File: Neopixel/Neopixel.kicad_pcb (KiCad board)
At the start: 2 copper layers, 22 parts

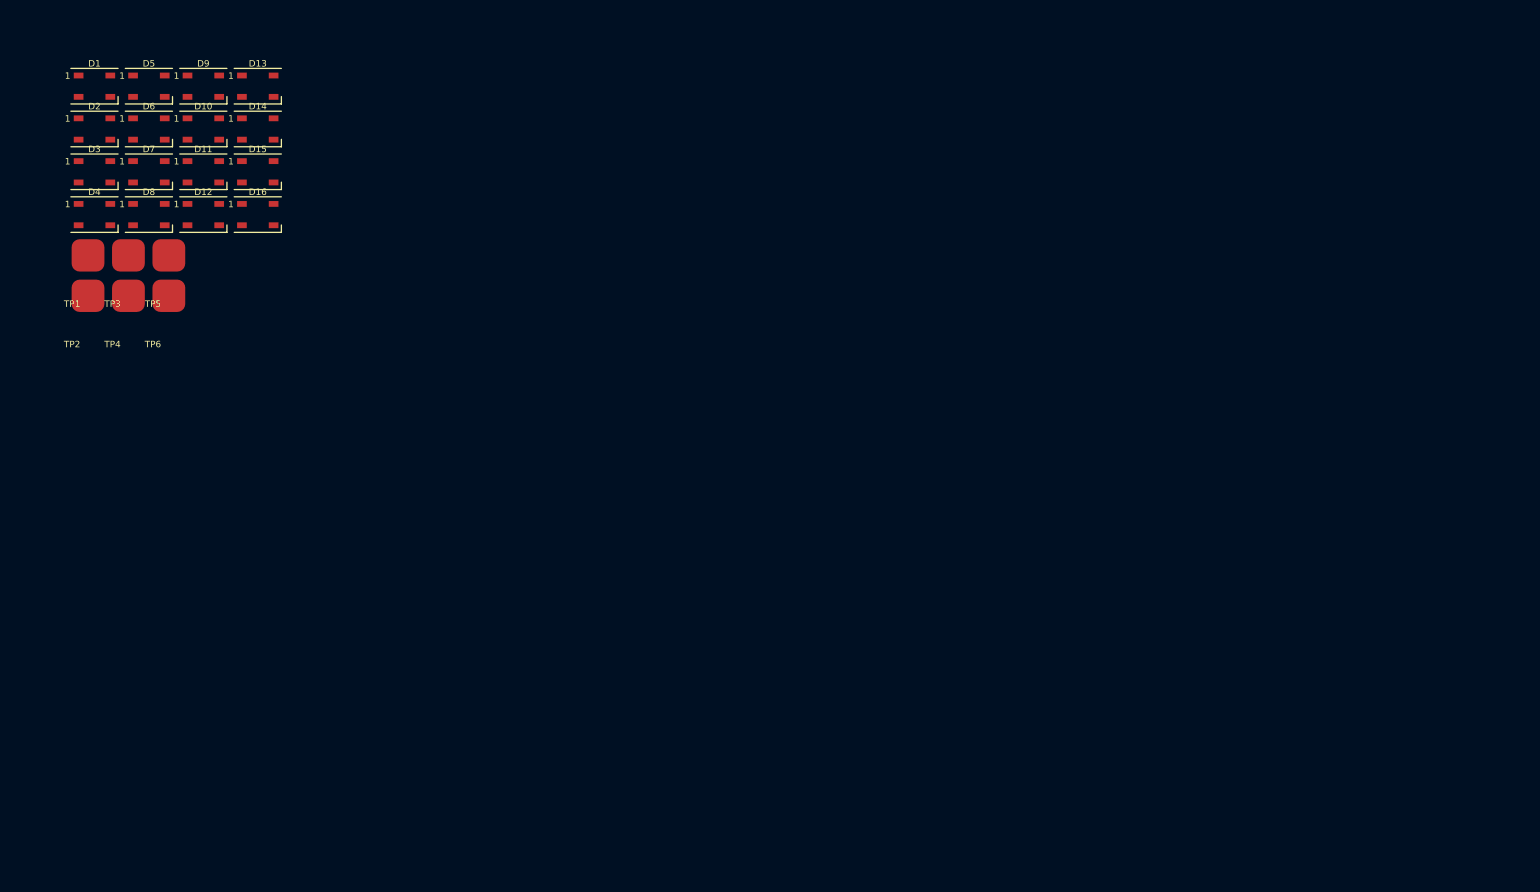
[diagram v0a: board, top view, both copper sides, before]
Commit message: designing
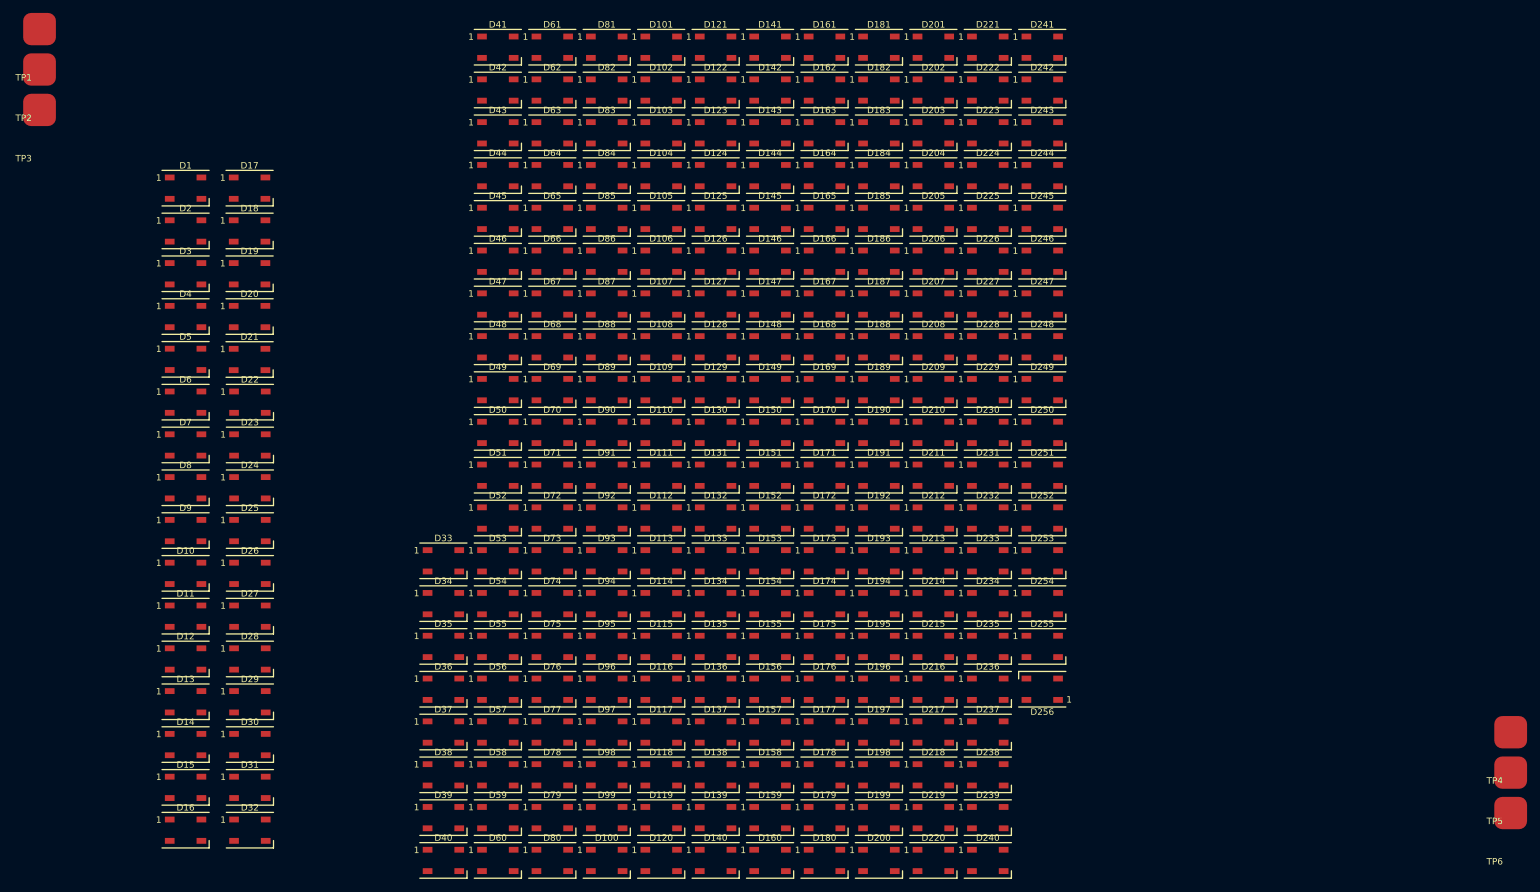
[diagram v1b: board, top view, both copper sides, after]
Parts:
- added D100: WS2812B, LED_SMD:LED_WS2812B_PLCC4_5.0x5.0mm_P3.2mm, F.Cu at (105.2, 147.3)
- added D101: WS2812B, LED_SMD:LED_WS2812B_PLCC4_5.0x5.0mm_P3.2mm, F.Cu at (113.6, 21.6)
- added D102: WS2812B, LED_SMD:LED_WS2812B_PLCC4_5.0x5.0mm_P3.2mm, F.Cu at (113.6, 28.2)
- added D103: WS2812B, LED_SMD:LED_WS2812B_PLCC4_5.0x5.0mm_P3.2mm, F.Cu at (113.6, 34.8)
- added D104: WS2812B, LED_SMD:LED_WS2812B_PLCC4_5.0x5.0mm_P3.2mm, F.Cu at (113.6, 41.4)
- added D105: WS2812B, LED_SMD:LED_WS2812B_PLCC4_5.0x5.0mm_P3.2mm, F.Cu at (113.6, 48.0)
- added D106: WS2812B, LED_SMD:LED_WS2812B_PLCC4_5.0x5.0mm_P3.2mm, F.Cu at (113.6, 54.6)
- added D107: WS2812B, LED_SMD:LED_WS2812B_PLCC4_5.0x5.0mm_P3.2mm, F.Cu at (113.6, 61.3)
- added D108: WS2812B, LED_SMD:LED_WS2812B_PLCC4_5.0x5.0mm_P3.2mm, F.Cu at (113.6, 67.9)
- added D109: WS2812B, LED_SMD:LED_WS2812B_PLCC4_5.0x5.0mm_P3.2mm, F.Cu at (113.6, 74.5)
- added D110: WS2812B, LED_SMD:LED_WS2812B_PLCC4_5.0x5.0mm_P3.2mm, F.Cu at (113.6, 81.1)
- added D111: WS2812B, LED_SMD:LED_WS2812B_PLCC4_5.0x5.0mm_P3.2mm, F.Cu at (113.6, 87.8)
- added D112: WS2812B, LED_SMD:LED_WS2812B_PLCC4_5.0x5.0mm_P3.2mm, F.Cu at (113.6, 94.4)
- added D113: WS2812B, LED_SMD:LED_WS2812B_PLCC4_5.0x5.0mm_P3.2mm, F.Cu at (113.6, 101.0)
- added D114: WS2812B, LED_SMD:LED_WS2812B_PLCC4_5.0x5.0mm_P3.2mm, F.Cu at (113.6, 107.6)
- added D115: WS2812B, LED_SMD:LED_WS2812B_PLCC4_5.0x5.0mm_P3.2mm, F.Cu at (113.6, 114.2)
- added D116: WS2812B, LED_SMD:LED_WS2812B_PLCC4_5.0x5.0mm_P3.2mm, F.Cu at (113.6, 120.8)
- added D117: WS2812B, LED_SMD:LED_WS2812B_PLCC4_5.0x5.0mm_P3.2mm, F.Cu at (113.6, 127.5)
- added D118: WS2812B, LED_SMD:LED_WS2812B_PLCC4_5.0x5.0mm_P3.2mm, F.Cu at (113.6, 134.1)
- added D119: WS2812B, LED_SMD:LED_WS2812B_PLCC4_5.0x5.0mm_P3.2mm, F.Cu at (113.6, 140.7)
- added D120: WS2812B, LED_SMD:LED_WS2812B_PLCC4_5.0x5.0mm_P3.2mm, F.Cu at (113.6, 147.3)
- added D121: WS2812B, LED_SMD:LED_WS2812B_PLCC4_5.0x5.0mm_P3.2mm, F.Cu at (122.0, 21.6)
- added D122: WS2812B, LED_SMD:LED_WS2812B_PLCC4_5.0x5.0mm_P3.2mm, F.Cu at (122.0, 28.2)
- added D123: WS2812B, LED_SMD:LED_WS2812B_PLCC4_5.0x5.0mm_P3.2mm, F.Cu at (122.0, 34.8)
- added D124: WS2812B, LED_SMD:LED_WS2812B_PLCC4_5.0x5.0mm_P3.2mm, F.Cu at (122.0, 41.4)
- added D125: WS2812B, LED_SMD:LED_WS2812B_PLCC4_5.0x5.0mm_P3.2mm, F.Cu at (122.0, 48.0)
- added D126: WS2812B, LED_SMD:LED_WS2812B_PLCC4_5.0x5.0mm_P3.2mm, F.Cu at (122.0, 54.6)
- added D127: WS2812B, LED_SMD:LED_WS2812B_PLCC4_5.0x5.0mm_P3.2mm, F.Cu at (122.0, 61.3)
- added D128: WS2812B, LED_SMD:LED_WS2812B_PLCC4_5.0x5.0mm_P3.2mm, F.Cu at (122.0, 67.9)
- added D129: WS2812B, LED_SMD:LED_WS2812B_PLCC4_5.0x5.0mm_P3.2mm, F.Cu at (122.0, 74.5)
- added D130: WS2812B, LED_SMD:LED_WS2812B_PLCC4_5.0x5.0mm_P3.2mm, F.Cu at (122.0, 81.1)
- added D131: WS2812B, LED_SMD:LED_WS2812B_PLCC4_5.0x5.0mm_P3.2mm, F.Cu at (122.0, 87.8)
- added D132: WS2812B, LED_SMD:LED_WS2812B_PLCC4_5.0x5.0mm_P3.2mm, F.Cu at (122.0, 94.4)
- added D133: WS2812B, LED_SMD:LED_WS2812B_PLCC4_5.0x5.0mm_P3.2mm, F.Cu at (122.0, 101.0)
- added D134: WS2812B, LED_SMD:LED_WS2812B_PLCC4_5.0x5.0mm_P3.2mm, F.Cu at (122.0, 107.6)
- added D135: WS2812B, LED_SMD:LED_WS2812B_PLCC4_5.0x5.0mm_P3.2mm, F.Cu at (122.0, 114.2)
- added D136: WS2812B, LED_SMD:LED_WS2812B_PLCC4_5.0x5.0mm_P3.2mm, F.Cu at (122.0, 120.8)
- added D137: WS2812B, LED_SMD:LED_WS2812B_PLCC4_5.0x5.0mm_P3.2mm, F.Cu at (122.0, 127.5)
- added D138: WS2812B, LED_SMD:LED_WS2812B_PLCC4_5.0x5.0mm_P3.2mm, F.Cu at (122.0, 134.1)
- added D139: WS2812B, LED_SMD:LED_WS2812B_PLCC4_5.0x5.0mm_P3.2mm, F.Cu at (122.0, 140.7)
- added D140: WS2812B, LED_SMD:LED_WS2812B_PLCC4_5.0x5.0mm_P3.2mm, F.Cu at (122.0, 147.3)
- added D141: WS2812B, LED_SMD:LED_WS2812B_PLCC4_5.0x5.0mm_P3.2mm, F.Cu at (130.4, 21.6)
- added D142: WS2812B, LED_SMD:LED_WS2812B_PLCC4_5.0x5.0mm_P3.2mm, F.Cu at (130.4, 28.2)
- added D143: WS2812B, LED_SMD:LED_WS2812B_PLCC4_5.0x5.0mm_P3.2mm, F.Cu at (130.4, 34.8)
- added D144: WS2812B, LED_SMD:LED_WS2812B_PLCC4_5.0x5.0mm_P3.2mm, F.Cu at (130.4, 41.4)
- added D145: WS2812B, LED_SMD:LED_WS2812B_PLCC4_5.0x5.0mm_P3.2mm, F.Cu at (130.4, 48.0)
- added D146: WS2812B, LED_SMD:LED_WS2812B_PLCC4_5.0x5.0mm_P3.2mm, F.Cu at (130.4, 54.6)
- added D147: WS2812B, LED_SMD:LED_WS2812B_PLCC4_5.0x5.0mm_P3.2mm, F.Cu at (130.4, 61.3)
- added D148: WS2812B, LED_SMD:LED_WS2812B_PLCC4_5.0x5.0mm_P3.2mm, F.Cu at (130.4, 67.9)
- added D149: WS2812B, LED_SMD:LED_WS2812B_PLCC4_5.0x5.0mm_P3.2mm, F.Cu at (130.4, 74.5)
- added D150: WS2812B, LED_SMD:LED_WS2812B_PLCC4_5.0x5.0mm_P3.2mm, F.Cu at (130.4, 81.1)
- added D151: WS2812B, LED_SMD:LED_WS2812B_PLCC4_5.0x5.0mm_P3.2mm, F.Cu at (130.4, 87.8)
- added D152: WS2812B, LED_SMD:LED_WS2812B_PLCC4_5.0x5.0mm_P3.2mm, F.Cu at (130.4, 94.4)
- added D153: WS2812B, LED_SMD:LED_WS2812B_PLCC4_5.0x5.0mm_P3.2mm, F.Cu at (130.4, 101.0)
- added D154: WS2812B, LED_SMD:LED_WS2812B_PLCC4_5.0x5.0mm_P3.2mm, F.Cu at (130.4, 107.6)
- added D155: WS2812B, LED_SMD:LED_WS2812B_PLCC4_5.0x5.0mm_P3.2mm, F.Cu at (130.4, 114.2)
- added D156: WS2812B, LED_SMD:LED_WS2812B_PLCC4_5.0x5.0mm_P3.2mm, F.Cu at (130.4, 120.8)
- added D157: WS2812B, LED_SMD:LED_WS2812B_PLCC4_5.0x5.0mm_P3.2mm, F.Cu at (130.4, 127.5)
- added D158: WS2812B, LED_SMD:LED_WS2812B_PLCC4_5.0x5.0mm_P3.2mm, F.Cu at (130.4, 134.1)
- added D159: WS2812B, LED_SMD:LED_WS2812B_PLCC4_5.0x5.0mm_P3.2mm, F.Cu at (130.4, 140.7)
- added D160: WS2812B, LED_SMD:LED_WS2812B_PLCC4_5.0x5.0mm_P3.2mm, F.Cu at (130.4, 147.3)
- added D161: WS2812B, LED_SMD:LED_WS2812B_PLCC4_5.0x5.0mm_P3.2mm, F.Cu at (138.9, 21.6)
- added D162: WS2812B, LED_SMD:LED_WS2812B_PLCC4_5.0x5.0mm_P3.2mm, F.Cu at (138.9, 28.2)
- added D163: WS2812B, LED_SMD:LED_WS2812B_PLCC4_5.0x5.0mm_P3.2mm, F.Cu at (138.9, 34.8)
- added D164: WS2812B, LED_SMD:LED_WS2812B_PLCC4_5.0x5.0mm_P3.2mm, F.Cu at (138.9, 41.4)
- added D165: WS2812B, LED_SMD:LED_WS2812B_PLCC4_5.0x5.0mm_P3.2mm, F.Cu at (138.9, 48.0)
- added D166: WS2812B, LED_SMD:LED_WS2812B_PLCC4_5.0x5.0mm_P3.2mm, F.Cu at (138.9, 54.6)
- added D167: WS2812B, LED_SMD:LED_WS2812B_PLCC4_5.0x5.0mm_P3.2mm, F.Cu at (138.9, 61.3)
- added D168: WS2812B, LED_SMD:LED_WS2812B_PLCC4_5.0x5.0mm_P3.2mm, F.Cu at (138.9, 67.9)
- added D169: WS2812B, LED_SMD:LED_WS2812B_PLCC4_5.0x5.0mm_P3.2mm, F.Cu at (138.9, 74.5)
- added D17: WS2812B, LED_SMD:LED_WS2812B_PLCC4_5.0x5.0mm_P3.2mm, F.Cu at (50.0, 43.4)
- added D170: WS2812B, LED_SMD:LED_WS2812B_PLCC4_5.0x5.0mm_P3.2mm, F.Cu at (138.9, 81.1)
- added D171: WS2812B, LED_SMD:LED_WS2812B_PLCC4_5.0x5.0mm_P3.2mm, F.Cu at (138.9, 87.8)
- added D172: WS2812B, LED_SMD:LED_WS2812B_PLCC4_5.0x5.0mm_P3.2mm, F.Cu at (138.9, 94.4)
- added D173: WS2812B, LED_SMD:LED_WS2812B_PLCC4_5.0x5.0mm_P3.2mm, F.Cu at (138.9, 101.0)
- added D174: WS2812B, LED_SMD:LED_WS2812B_PLCC4_5.0x5.0mm_P3.2mm, F.Cu at (138.9, 107.6)
- added D175: WS2812B, LED_SMD:LED_WS2812B_PLCC4_5.0x5.0mm_P3.2mm, F.Cu at (138.9, 114.2)
- added D176: WS2812B, LED_SMD:LED_WS2812B_PLCC4_5.0x5.0mm_P3.2mm, F.Cu at (138.9, 120.8)
- added D177: WS2812B, LED_SMD:LED_WS2812B_PLCC4_5.0x5.0mm_P3.2mm, F.Cu at (138.9, 127.5)
- added D178: WS2812B, LED_SMD:LED_WS2812B_PLCC4_5.0x5.0mm_P3.2mm, F.Cu at (138.9, 134.1)
- added D179: WS2812B, LED_SMD:LED_WS2812B_PLCC4_5.0x5.0mm_P3.2mm, F.Cu at (138.9, 140.7)
- added D18: WS2812B, LED_SMD:LED_WS2812B_PLCC4_5.0x5.0mm_P3.2mm, F.Cu at (50.0, 50.0)
- added D180: WS2812B, LED_SMD:LED_WS2812B_PLCC4_5.0x5.0mm_P3.2mm, F.Cu at (138.9, 147.3)
- added D181: WS2812B, LED_SMD:LED_WS2812B_PLCC4_5.0x5.0mm_P3.2mm, F.Cu at (147.3, 21.6)
- added D182: WS2812B, LED_SMD:LED_WS2812B_PLCC4_5.0x5.0mm_P3.2mm, F.Cu at (147.3, 28.2)
- added D183: WS2812B, LED_SMD:LED_WS2812B_PLCC4_5.0x5.0mm_P3.2mm, F.Cu at (147.3, 34.8)
- added D184: WS2812B, LED_SMD:LED_WS2812B_PLCC4_5.0x5.0mm_P3.2mm, F.Cu at (147.3, 41.4)
- added D185: WS2812B, LED_SMD:LED_WS2812B_PLCC4_5.0x5.0mm_P3.2mm, F.Cu at (147.3, 48.0)
- added D186: WS2812B, LED_SMD:LED_WS2812B_PLCC4_5.0x5.0mm_P3.2mm, F.Cu at (147.3, 54.6)
- added D187: WS2812B, LED_SMD:LED_WS2812B_PLCC4_5.0x5.0mm_P3.2mm, F.Cu at (147.3, 61.3)
- added D188: WS2812B, LED_SMD:LED_WS2812B_PLCC4_5.0x5.0mm_P3.2mm, F.Cu at (147.3, 67.9)
- added D189: WS2812B, LED_SMD:LED_WS2812B_PLCC4_5.0x5.0mm_P3.2mm, F.Cu at (147.3, 74.5)
- added D19: WS2812B, LED_SMD:LED_WS2812B_PLCC4_5.0x5.0mm_P3.2mm, F.Cu at (50.0, 56.6)
- added D190: WS2812B, LED_SMD:LED_WS2812B_PLCC4_5.0x5.0mm_P3.2mm, F.Cu at (147.3, 81.1)
- added D191: WS2812B, LED_SMD:LED_WS2812B_PLCC4_5.0x5.0mm_P3.2mm, F.Cu at (147.3, 87.8)
- added D192: WS2812B, LED_SMD:LED_WS2812B_PLCC4_5.0x5.0mm_P3.2mm, F.Cu at (147.3, 94.4)
- added D193: WS2812B, LED_SMD:LED_WS2812B_PLCC4_5.0x5.0mm_P3.2mm, F.Cu at (147.3, 101.0)
- added D194: WS2812B, LED_SMD:LED_WS2812B_PLCC4_5.0x5.0mm_P3.2mm, F.Cu at (147.3, 107.6)
- added D195: WS2812B, LED_SMD:LED_WS2812B_PLCC4_5.0x5.0mm_P3.2mm, F.Cu at (147.3, 114.2)
- added D196: WS2812B, LED_SMD:LED_WS2812B_PLCC4_5.0x5.0mm_P3.2mm, F.Cu at (147.3, 120.8)
- added D197: WS2812B, LED_SMD:LED_WS2812B_PLCC4_5.0x5.0mm_P3.2mm, F.Cu at (147.3, 127.5)
- added D198: WS2812B, LED_SMD:LED_WS2812B_PLCC4_5.0x5.0mm_P3.2mm, F.Cu at (147.3, 134.1)
- added D199: WS2812B, LED_SMD:LED_WS2812B_PLCC4_5.0x5.0mm_P3.2mm, F.Cu at (147.3, 140.7)
- added D20: WS2812B, LED_SMD:LED_WS2812B_PLCC4_5.0x5.0mm_P3.2mm, F.Cu at (50.0, 63.2)
- added D200: WS2812B, LED_SMD:LED_WS2812B_PLCC4_5.0x5.0mm_P3.2mm, F.Cu at (147.3, 147.3)
- added D201: WS2812B, LED_SMD:LED_WS2812B_PLCC4_5.0x5.0mm_P3.2mm, F.Cu at (155.7, 21.6)
- added D202: WS2812B, LED_SMD:LED_WS2812B_PLCC4_5.0x5.0mm_P3.2mm, F.Cu at (155.7, 28.2)
- added D203: WS2812B, LED_SMD:LED_WS2812B_PLCC4_5.0x5.0mm_P3.2mm, F.Cu at (155.7, 34.8)
- added D204: WS2812B, LED_SMD:LED_WS2812B_PLCC4_5.0x5.0mm_P3.2mm, F.Cu at (155.7, 41.4)
- added D205: WS2812B, LED_SMD:LED_WS2812B_PLCC4_5.0x5.0mm_P3.2mm, F.Cu at (155.7, 48.0)
- added D206: WS2812B, LED_SMD:LED_WS2812B_PLCC4_5.0x5.0mm_P3.2mm, F.Cu at (155.7, 54.6)
- added D207: WS2812B, LED_SMD:LED_WS2812B_PLCC4_5.0x5.0mm_P3.2mm, F.Cu at (155.7, 61.3)
- added D208: WS2812B, LED_SMD:LED_WS2812B_PLCC4_5.0x5.0mm_P3.2mm, F.Cu at (155.7, 67.9)
- added D209: WS2812B, LED_SMD:LED_WS2812B_PLCC4_5.0x5.0mm_P3.2mm, F.Cu at (155.7, 74.5)
- added D21: WS2812B, LED_SMD:LED_WS2812B_PLCC4_5.0x5.0mm_P3.2mm, F.Cu at (50.0, 69.8)
- added D210: WS2812B, LED_SMD:LED_WS2812B_PLCC4_5.0x5.0mm_P3.2mm, F.Cu at (155.7, 81.1)
- added D211: WS2812B, LED_SMD:LED_WS2812B_PLCC4_5.0x5.0mm_P3.2mm, F.Cu at (155.7, 87.8)
- added D212: WS2812B, LED_SMD:LED_WS2812B_PLCC4_5.0x5.0mm_P3.2mm, F.Cu at (155.7, 94.4)
- added D213: WS2812B, LED_SMD:LED_WS2812B_PLCC4_5.0x5.0mm_P3.2mm, F.Cu at (155.7, 101.0)
- added D214: WS2812B, LED_SMD:LED_WS2812B_PLCC4_5.0x5.0mm_P3.2mm, F.Cu at (155.7, 107.6)
- added D215: WS2812B, LED_SMD:LED_WS2812B_PLCC4_5.0x5.0mm_P3.2mm, F.Cu at (155.7, 114.2)
- added D216: WS2812B, LED_SMD:LED_WS2812B_PLCC4_5.0x5.0mm_P3.2mm, F.Cu at (155.7, 120.8)
- added D217: WS2812B, LED_SMD:LED_WS2812B_PLCC4_5.0x5.0mm_P3.2mm, F.Cu at (155.7, 127.5)
- added D218: WS2812B, LED_SMD:LED_WS2812B_PLCC4_5.0x5.0mm_P3.2mm, F.Cu at (155.7, 134.1)
- added D219: WS2812B, LED_SMD:LED_WS2812B_PLCC4_5.0x5.0mm_P3.2mm, F.Cu at (155.7, 140.7)
- added D22: WS2812B, LED_SMD:LED_WS2812B_PLCC4_5.0x5.0mm_P3.2mm, F.Cu at (50.0, 76.5)
- added D220: WS2812B, LED_SMD:LED_WS2812B_PLCC4_5.0x5.0mm_P3.2mm, F.Cu at (155.7, 147.3)
- added D221: WS2812B, LED_SMD:LED_WS2812B_PLCC4_5.0x5.0mm_P3.2mm, F.Cu at (164.1, 21.6)
- added D222: WS2812B, LED_SMD:LED_WS2812B_PLCC4_5.0x5.0mm_P3.2mm, F.Cu at (164.1, 28.2)
- added D223: WS2812B, LED_SMD:LED_WS2812B_PLCC4_5.0x5.0mm_P3.2mm, F.Cu at (164.1, 34.8)
- added D224: WS2812B, LED_SMD:LED_WS2812B_PLCC4_5.0x5.0mm_P3.2mm, F.Cu at (164.1, 41.4)
- added D225: WS2812B, LED_SMD:LED_WS2812B_PLCC4_5.0x5.0mm_P3.2mm, F.Cu at (164.1, 48.0)
- added D226: WS2812B, LED_SMD:LED_WS2812B_PLCC4_5.0x5.0mm_P3.2mm, F.Cu at (164.1, 54.6)
- added D227: WS2812B, LED_SMD:LED_WS2812B_PLCC4_5.0x5.0mm_P3.2mm, F.Cu at (164.1, 61.3)
- added D228: WS2812B, LED_SMD:LED_WS2812B_PLCC4_5.0x5.0mm_P3.2mm, F.Cu at (164.1, 67.9)
- added D229: WS2812B, LED_SMD:LED_WS2812B_PLCC4_5.0x5.0mm_P3.2mm, F.Cu at (164.1, 74.5)
- added D23: WS2812B, LED_SMD:LED_WS2812B_PLCC4_5.0x5.0mm_P3.2mm, F.Cu at (50.0, 83.1)
- added D230: WS2812B, LED_SMD:LED_WS2812B_PLCC4_5.0x5.0mm_P3.2mm, F.Cu at (164.1, 81.1)
- added D231: WS2812B, LED_SMD:LED_WS2812B_PLCC4_5.0x5.0mm_P3.2mm, F.Cu at (164.1, 87.8)
- added D232: WS2812B, LED_SMD:LED_WS2812B_PLCC4_5.0x5.0mm_P3.2mm, F.Cu at (164.1, 94.4)
- added D233: WS2812B, LED_SMD:LED_WS2812B_PLCC4_5.0x5.0mm_P3.2mm, F.Cu at (164.1, 101.0)
- added D234: WS2812B, LED_SMD:LED_WS2812B_PLCC4_5.0x5.0mm_P3.2mm, F.Cu at (164.1, 107.6)
- added D235: WS2812B, LED_SMD:LED_WS2812B_PLCC4_5.0x5.0mm_P3.2mm, F.Cu at (164.1, 114.2)
- added D236: WS2812B, LED_SMD:LED_WS2812B_PLCC4_5.0x5.0mm_P3.2mm, F.Cu at (164.1, 120.8)
- added D237: WS2812B, LED_SMD:LED_WS2812B_PLCC4_5.0x5.0mm_P3.2mm, F.Cu at (164.1, 127.5)
- added D238: WS2812B, LED_SMD:LED_WS2812B_PLCC4_5.0x5.0mm_P3.2mm, F.Cu at (164.1, 134.1)
- added D239: WS2812B, LED_SMD:LED_WS2812B_PLCC4_5.0x5.0mm_P3.2mm, F.Cu at (164.1, 140.7)
- added D24: WS2812B, LED_SMD:LED_WS2812B_PLCC4_5.0x5.0mm_P3.2mm, F.Cu at (50.0, 89.7)
- added D240: WS2812B, LED_SMD:LED_WS2812B_PLCC4_5.0x5.0mm_P3.2mm, F.Cu at (164.1, 147.3)
- added D241: WS2812B, LED_SMD:LED_WS2812B_PLCC4_5.0x5.0mm_P3.2mm, F.Cu at (172.6, 21.6)
- added D242: WS2812B, LED_SMD:LED_WS2812B_PLCC4_5.0x5.0mm_P3.2mm, F.Cu at (172.6, 28.2)
- added D243: WS2812B, LED_SMD:LED_WS2812B_PLCC4_5.0x5.0mm_P3.2mm, F.Cu at (172.6, 34.8)
- added D244: WS2812B, LED_SMD:LED_WS2812B_PLCC4_5.0x5.0mm_P3.2mm, F.Cu at (172.6, 41.4)
- added D245: WS2812B, LED_SMD:LED_WS2812B_PLCC4_5.0x5.0mm_P3.2mm, F.Cu at (172.6, 48.0)
- added D246: WS2812B, LED_SMD:LED_WS2812B_PLCC4_5.0x5.0mm_P3.2mm, F.Cu at (172.6, 54.6)
- added D247: WS2812B, LED_SMD:LED_WS2812B_PLCC4_5.0x5.0mm_P3.2mm, F.Cu at (172.6, 61.3)
- added D248: WS2812B, LED_SMD:LED_WS2812B_PLCC4_5.0x5.0mm_P3.2mm, F.Cu at (172.6, 67.9)
- added D249: WS2812B, LED_SMD:LED_WS2812B_PLCC4_5.0x5.0mm_P3.2mm, F.Cu at (172.6, 74.5)
- added D25: WS2812B, LED_SMD:LED_WS2812B_PLCC4_5.0x5.0mm_P3.2mm, F.Cu at (50.0, 96.3)
- added D250: WS2812B, LED_SMD:LED_WS2812B_PLCC4_5.0x5.0mm_P3.2mm, F.Cu at (172.6, 81.1)
- added D251: WS2812B, LED_SMD:LED_WS2812B_PLCC4_5.0x5.0mm_P3.2mm, F.Cu at (172.6, 87.8)
- added D252: WS2812B, LED_SMD:LED_WS2812B_PLCC4_5.0x5.0mm_P3.2mm, F.Cu at (172.6, 94.4)
- added D253: WS2812B, LED_SMD:LED_WS2812B_PLCC4_5.0x5.0mm_P3.2mm, F.Cu at (172.6, 101.0)
- added D254: WS2812B, LED_SMD:LED_WS2812B_PLCC4_5.0x5.0mm_P3.2mm, F.Cu at (172.6, 107.6)
- added D255: WS2812B, LED_SMD:LED_WS2812B_PLCC4_5.0x5.0mm_P3.2mm, F.Cu at (172.6, 114.2)
- added D256: WS2812B, LED_SMD:LED_WS2812B_PLCC4_5.0x5.0mm_P3.2mm, F.Cu at (172.6, 120.8)
- added D26: WS2812B, LED_SMD:LED_WS2812B_PLCC4_5.0x5.0mm_P3.2mm, F.Cu at (50.0, 102.9)
- added D27: WS2812B, LED_SMD:LED_WS2812B_PLCC4_5.0x5.0mm_P3.2mm, F.Cu at (50.0, 109.5)
- added D28: WS2812B, LED_SMD:LED_WS2812B_PLCC4_5.0x5.0mm_P3.2mm, F.Cu at (50.0, 116.2)
- added D29: WS2812B, LED_SMD:LED_WS2812B_PLCC4_5.0x5.0mm_P3.2mm, F.Cu at (50.0, 122.8)
- added D30: WS2812B, LED_SMD:LED_WS2812B_PLCC4_5.0x5.0mm_P3.2mm, F.Cu at (50.0, 129.4)
- added D31: WS2812B, LED_SMD:LED_WS2812B_PLCC4_5.0x5.0mm_P3.2mm, F.Cu at (50.0, 136.0)
- added D32: WS2812B, LED_SMD:LED_WS2812B_PLCC4_5.0x5.0mm_P3.2mm, F.Cu at (50.0, 142.7)
- added D33: WS2812B, LED_SMD:LED_WS2812B_PLCC4_5.0x5.0mm_P3.2mm, F.Cu at (79.9, 101.0)
- added D34: WS2812B, LED_SMD:LED_WS2812B_PLCC4_5.0x5.0mm_P3.2mm, F.Cu at (79.9, 107.6)
- added D35: WS2812B, LED_SMD:LED_WS2812B_PLCC4_5.0x5.0mm_P3.2mm, F.Cu at (79.9, 114.2)
- added D36: WS2812B, LED_SMD:LED_WS2812B_PLCC4_5.0x5.0mm_P3.2mm, F.Cu at (79.9, 120.8)
- added D37: WS2812B, LED_SMD:LED_WS2812B_PLCC4_5.0x5.0mm_P3.2mm, F.Cu at (79.9, 127.5)
- added D38: WS2812B, LED_SMD:LED_WS2812B_PLCC4_5.0x5.0mm_P3.2mm, F.Cu at (79.9, 134.1)
- added D39: WS2812B, LED_SMD:LED_WS2812B_PLCC4_5.0x5.0mm_P3.2mm, F.Cu at (79.9, 140.7)
- added D40: WS2812B, LED_SMD:LED_WS2812B_PLCC4_5.0x5.0mm_P3.2mm, F.Cu at (79.9, 147.3)
- added D41: WS2812B, LED_SMD:LED_WS2812B_PLCC4_5.0x5.0mm_P3.2mm, F.Cu at (88.3, 21.6)
- added D42: WS2812B, LED_SMD:LED_WS2812B_PLCC4_5.0x5.0mm_P3.2mm, F.Cu at (88.3, 28.2)
- added D43: WS2812B, LED_SMD:LED_WS2812B_PLCC4_5.0x5.0mm_P3.2mm, F.Cu at (88.3, 34.8)
- added D44: WS2812B, LED_SMD:LED_WS2812B_PLCC4_5.0x5.0mm_P3.2mm, F.Cu at (88.3, 41.4)
- added D45: WS2812B, LED_SMD:LED_WS2812B_PLCC4_5.0x5.0mm_P3.2mm, F.Cu at (88.3, 48.0)
- added D46: WS2812B, LED_SMD:LED_WS2812B_PLCC4_5.0x5.0mm_P3.2mm, F.Cu at (88.3, 54.6)
- added D47: WS2812B, LED_SMD:LED_WS2812B_PLCC4_5.0x5.0mm_P3.2mm, F.Cu at (88.3, 61.3)
- added D48: WS2812B, LED_SMD:LED_WS2812B_PLCC4_5.0x5.0mm_P3.2mm, F.Cu at (88.3, 67.9)
- added D49: WS2812B, LED_SMD:LED_WS2812B_PLCC4_5.0x5.0mm_P3.2mm, F.Cu at (88.3, 74.5)
- added D50: WS2812B, LED_SMD:LED_WS2812B_PLCC4_5.0x5.0mm_P3.2mm, F.Cu at (88.3, 81.1)
- added D51: WS2812B, LED_SMD:LED_WS2812B_PLCC4_5.0x5.0mm_P3.2mm, F.Cu at (88.3, 87.8)
- added D52: WS2812B, LED_SMD:LED_WS2812B_PLCC4_5.0x5.0mm_P3.2mm, F.Cu at (88.3, 94.4)
- added D53: WS2812B, LED_SMD:LED_WS2812B_PLCC4_5.0x5.0mm_P3.2mm, F.Cu at (88.3, 101.0)
- added D54: WS2812B, LED_SMD:LED_WS2812B_PLCC4_5.0x5.0mm_P3.2mm, F.Cu at (88.3, 107.6)
- added D55: WS2812B, LED_SMD:LED_WS2812B_PLCC4_5.0x5.0mm_P3.2mm, F.Cu at (88.3, 114.2)
- added D56: WS2812B, LED_SMD:LED_WS2812B_PLCC4_5.0x5.0mm_P3.2mm, F.Cu at (88.3, 120.8)
- added D57: WS2812B, LED_SMD:LED_WS2812B_PLCC4_5.0x5.0mm_P3.2mm, F.Cu at (88.3, 127.5)
- added D58: WS2812B, LED_SMD:LED_WS2812B_PLCC4_5.0x5.0mm_P3.2mm, F.Cu at (88.3, 134.1)
- added D59: WS2812B, LED_SMD:LED_WS2812B_PLCC4_5.0x5.0mm_P3.2mm, F.Cu at (88.3, 140.7)
- added D60: WS2812B, LED_SMD:LED_WS2812B_PLCC4_5.0x5.0mm_P3.2mm, F.Cu at (88.3, 147.3)
- added D61: WS2812B, LED_SMD:LED_WS2812B_PLCC4_5.0x5.0mm_P3.2mm, F.Cu at (96.8, 21.6)
- added D62: WS2812B, LED_SMD:LED_WS2812B_PLCC4_5.0x5.0mm_P3.2mm, F.Cu at (96.8, 28.2)
- added D63: WS2812B, LED_SMD:LED_WS2812B_PLCC4_5.0x5.0mm_P3.2mm, F.Cu at (96.8, 34.8)
- added D64: WS2812B, LED_SMD:LED_WS2812B_PLCC4_5.0x5.0mm_P3.2mm, F.Cu at (96.8, 41.4)
- added D65: WS2812B, LED_SMD:LED_WS2812B_PLCC4_5.0x5.0mm_P3.2mm, F.Cu at (96.8, 48.0)
- added D66: WS2812B, LED_SMD:LED_WS2812B_PLCC4_5.0x5.0mm_P3.2mm, F.Cu at (96.8, 54.6)
- added D67: WS2812B, LED_SMD:LED_WS2812B_PLCC4_5.0x5.0mm_P3.2mm, F.Cu at (96.8, 61.3)
- added D68: WS2812B, LED_SMD:LED_WS2812B_PLCC4_5.0x5.0mm_P3.2mm, F.Cu at (96.8, 67.9)
- added D69: WS2812B, LED_SMD:LED_WS2812B_PLCC4_5.0x5.0mm_P3.2mm, F.Cu at (96.8, 74.5)
- added D70: WS2812B, LED_SMD:LED_WS2812B_PLCC4_5.0x5.0mm_P3.2mm, F.Cu at (96.8, 81.1)
- added D71: WS2812B, LED_SMD:LED_WS2812B_PLCC4_5.0x5.0mm_P3.2mm, F.Cu at (96.8, 87.8)
- added D72: WS2812B, LED_SMD:LED_WS2812B_PLCC4_5.0x5.0mm_P3.2mm, F.Cu at (96.8, 94.4)
- added D73: WS2812B, LED_SMD:LED_WS2812B_PLCC4_5.0x5.0mm_P3.2mm, F.Cu at (96.8, 101.0)
- added D74: WS2812B, LED_SMD:LED_WS2812B_PLCC4_5.0x5.0mm_P3.2mm, F.Cu at (96.8, 107.6)
- added D75: WS2812B, LED_SMD:LED_WS2812B_PLCC4_5.0x5.0mm_P3.2mm, F.Cu at (96.8, 114.2)
- added D76: WS2812B, LED_SMD:LED_WS2812B_PLCC4_5.0x5.0mm_P3.2mm, F.Cu at (96.8, 120.8)
- added D77: WS2812B, LED_SMD:LED_WS2812B_PLCC4_5.0x5.0mm_P3.2mm, F.Cu at (96.8, 127.5)
- added D78: WS2812B, LED_SMD:LED_WS2812B_PLCC4_5.0x5.0mm_P3.2mm, F.Cu at (96.8, 134.1)
- added D79: WS2812B, LED_SMD:LED_WS2812B_PLCC4_5.0x5.0mm_P3.2mm, F.Cu at (96.8, 140.7)
- added D80: WS2812B, LED_SMD:LED_WS2812B_PLCC4_5.0x5.0mm_P3.2mm, F.Cu at (96.8, 147.3)
- added D81: WS2812B, LED_SMD:LED_WS2812B_PLCC4_5.0x5.0mm_P3.2mm, F.Cu at (105.2, 21.6)
- added D82: WS2812B, LED_SMD:LED_WS2812B_PLCC4_5.0x5.0mm_P3.2mm, F.Cu at (105.2, 28.2)
- added D83: WS2812B, LED_SMD:LED_WS2812B_PLCC4_5.0x5.0mm_P3.2mm, F.Cu at (105.2, 34.8)
- added D84: WS2812B, LED_SMD:LED_WS2812B_PLCC4_5.0x5.0mm_P3.2mm, F.Cu at (105.2, 41.4)
- added D85: WS2812B, LED_SMD:LED_WS2812B_PLCC4_5.0x5.0mm_P3.2mm, F.Cu at (105.2, 48.0)
- added D86: WS2812B, LED_SMD:LED_WS2812B_PLCC4_5.0x5.0mm_P3.2mm, F.Cu at (105.2, 54.6)
- added D87: WS2812B, LED_SMD:LED_WS2812B_PLCC4_5.0x5.0mm_P3.2mm, F.Cu at (105.2, 61.3)
- added D88: WS2812B, LED_SMD:LED_WS2812B_PLCC4_5.0x5.0mm_P3.2mm, F.Cu at (105.2, 67.9)
- added D89: WS2812B, LED_SMD:LED_WS2812B_PLCC4_5.0x5.0mm_P3.2mm, F.Cu at (105.2, 74.5)
- added D90: WS2812B, LED_SMD:LED_WS2812B_PLCC4_5.0x5.0mm_P3.2mm, F.Cu at (105.2, 81.1)
- added D91: WS2812B, LED_SMD:LED_WS2812B_PLCC4_5.0x5.0mm_P3.2mm, F.Cu at (105.2, 87.8)
- added D92: WS2812B, LED_SMD:LED_WS2812B_PLCC4_5.0x5.0mm_P3.2mm, F.Cu at (105.2, 94.4)
- added D93: WS2812B, LED_SMD:LED_WS2812B_PLCC4_5.0x5.0mm_P3.2mm, F.Cu at (105.2, 101.0)
- added D94: WS2812B, LED_SMD:LED_WS2812B_PLCC4_5.0x5.0mm_P3.2mm, F.Cu at (105.2, 107.6)
- added D95: WS2812B, LED_SMD:LED_WS2812B_PLCC4_5.0x5.0mm_P3.2mm, F.Cu at (105.2, 114.2)
- added D96: WS2812B, LED_SMD:LED_WS2812B_PLCC4_5.0x5.0mm_P3.2mm, F.Cu at (105.2, 120.8)
- added D97: WS2812B, LED_SMD:LED_WS2812B_PLCC4_5.0x5.0mm_P3.2mm, F.Cu at (105.2, 127.5)
- added D98: WS2812B, LED_SMD:LED_WS2812B_PLCC4_5.0x5.0mm_P3.2mm, F.Cu at (105.2, 134.1)
- added D99: WS2812B, LED_SMD:LED_WS2812B_PLCC4_5.0x5.0mm_P3.2mm, F.Cu at (105.2, 140.7)
- moved TP4 224.2 mm to (242.5, 130.0)
- moved TP5 222.4 mm to (242.5, 136.2)
- moved TP6 222.4 mm to (242.5, 142.5)
- moved D13 95.9 mm to (40.0, 122.8)
- moved D15 95.9 mm to (40.0, 136.0)
- moved D16 95.9 mm to (40.0, 142.7)
- moved D14 95.9 mm to (40.0, 129.4)
- moved D10 68.8 mm to (40.0, 102.9)
- moved D12 68.8 mm to (40.0, 116.2)
- moved D9 68.8 mm to (40.0, 96.3)
- moved D11 68.8 mm to (40.0, 109.5)
- moved D5 42.6 mm to (40.0, 69.8)
- moved D6 42.6 mm to (40.0, 76.5)
- moved D8 42.6 mm to (40.0, 89.7)
- moved D7 42.6 mm to (40.0, 83.1)
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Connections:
- TP4 pad 1: GND -> +5V
- TP5 pad 1: +5V -> GND
- TP6 pad 1: Net-(D16-DOUT) -> unconnected-(TP6-Pad1)

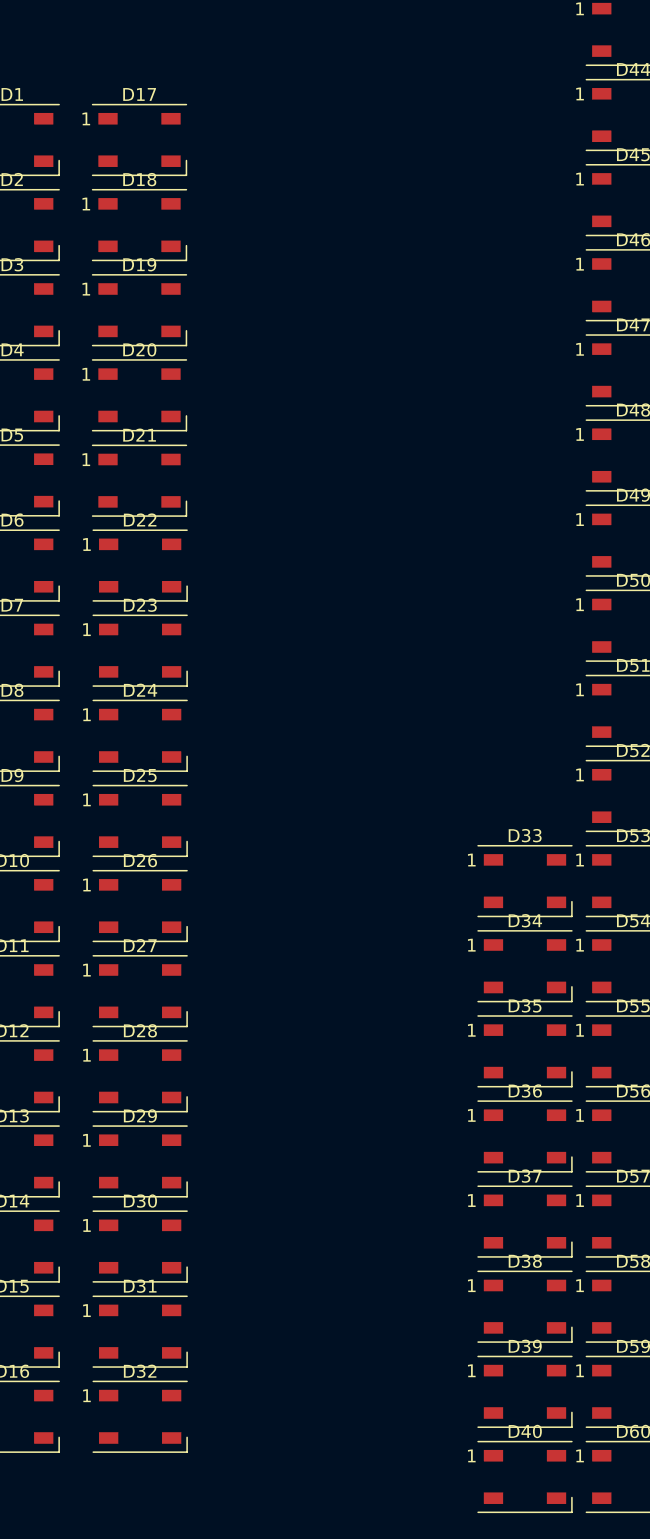
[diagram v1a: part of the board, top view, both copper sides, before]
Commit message: designing
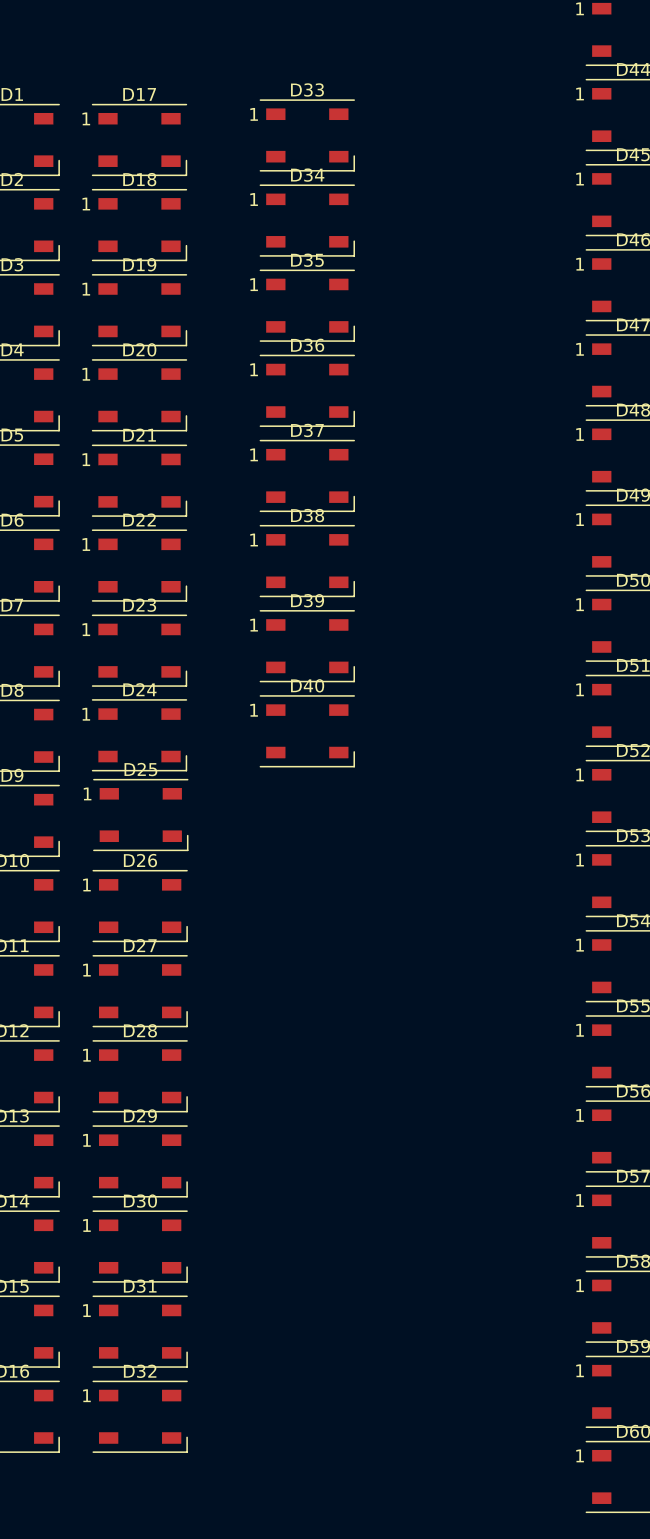
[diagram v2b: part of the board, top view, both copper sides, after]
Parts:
- moved D38 60.4 mm to (63.0, 76.1)
- moved D39 60.4 mm to (63.0, 82.7)
- moved D40 60.4 mm to (63.0, 89.3)
- moved D34 60.4 mm to (63.0, 49.6)
- moved D35 60.4 mm to (63.0, 56.2)
- moved D33 60.4 mm to (63.0, 43.0)
- moved D36 60.4 mm to (63.0, 62.9)
- moved D37 60.4 mm to (63.0, 69.5)
- moved D25 0.46 mm to (50.0, 95.8)
- moved D24 0.06 mm to (50.0, 89.7)
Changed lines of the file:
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@@
 	(footprint "LED_SMD:LED_WS2812B_PLCC4_5.0x5.0mm_P3.2mm"
 		(layer "F.Cu")
-		(at 79.93 120.85)
+		(at 63 62.86)
 		(descr "5.0mm x 5.0mm Addressable RGB LED NeoPixel, https://cdn-shop.adafruit.com/datasheets/WS2812B.pdf")
 		(tags "LED RGB NeoPixel PLCC-4 5050")
@@
 	(footprint "LED_SMD:LED_WS2812B_PLCC4_5.0x5.0mm_P3.2mm"
 		(layer "F.Cu")
-		(at 79.93 114.23)
+		(at 63 56.24)
 		(descr "5.0mm x 5.0mm Addressable RGB LED NeoPixel, https://cdn-shop.adafruit.com/datasheets/WS2812B.pdf")
 		(tags "LED RGB NeoPixel PLCC-4 5050")
@@
 	(footprint "LED_SMD:LED_WS2812B_PLCC4_5.0x5.0mm_P3.2mm"
 		(layer "F.Cu")
-		(at 50 83.07)
+		(at 49.95 83.07)
 		(descr "5.0mm x 5.0mm Addressable RGB LED NeoPixel, https://cdn-shop.adafruit.com/datasheets/WS2812B.pdf")
 		(tags "LED RGB NeoPixel PLCC-4 5050")
@@
 	(footprint "LED_SMD:LED_WS2812B_PLCC4_5.0x5.0mm_P3.2mm"
 		(layer "F.Cu")
-		(at 79.93 140.71)
+		(at 63 82.72)
 		(descr "5.0mm x 5.0mm Addressable RGB LED NeoPixel, https://cdn-shop.adafruit.com/datasheets/WS2812B.pdf")
 		(tags "LED RGB NeoPixel PLCC-4 5050")
@@
 	(footprint "LED_SMD:LED_WS2812B_PLCC4_5.0x5.0mm_P3.2mm"
 		(layer "F.Cu")
-		(at 50 89.69)
+		(at 49.95 89.65)
 		(descr "5.0mm x 5.0mm Addressable RGB LED NeoPixel, https://cdn-shop.adafruit.com/datasheets/WS2812B.pdf")
 		(tags "LED RGB NeoPixel PLCC-4 5050")
@@
 	(footprint "LED_SMD:LED_WS2812B_PLCC4_5.0x5.0mm_P3.2mm"
 		(layer "F.Cu")
-		(at 79.93 100.99)
+		(at 63 43)
 		(descr "5.0mm x 5.0mm Addressable RGB LED NeoPixel, https://cdn-shop.adafruit.com/datasheets/WS2812B.pdf")
 		(tags "LED RGB NeoPixel PLCC-4 5050")
@@
 	(footprint "LED_SMD:LED_WS2812B_PLCC4_5.0x5.0mm_P3.2mm"
 		(layer "F.Cu")
-		(at 79.93 134.09)
+		(at 63 76.1)
 		(descr "5.0mm x 5.0mm Addressable RGB LED NeoPixel, https://cdn-shop.adafruit.com/datasheets/WS2812B.pdf")
 		(tags "LED RGB NeoPixel PLCC-4 5050")
@@
 	(footprint "LED_SMD:LED_WS2812B_PLCC4_5.0x5.0mm_P3.2mm"
 		(layer "F.Cu")
-		(at 50 76.45)
+		(at 49.95 76.45)
 		(descr "5.0mm x 5.0mm Addressable RGB LED NeoPixel, https://cdn-shop.adafruit.com/datasheets/WS2812B.pdf")
 		(tags "LED RGB NeoPixel PLCC-4 5050")
@@
 	(footprint "LED_SMD:LED_WS2812B_PLCC4_5.0x5.0mm_P3.2mm"
 		(layer "F.Cu")
-		(at 50 96.31)
+		(at 50.05 95.85)
 		(descr "5.0mm x 5.0mm Addressable RGB LED NeoPixel, https://cdn-shop.adafruit.com/datasheets/WS2812B.pdf")
 		(tags "LED RGB NeoPixel PLCC-4 5050")
@@
 	(footprint "LED_SMD:LED_WS2812B_PLCC4_5.0x5.0mm_P3.2mm"
 		(layer "F.Cu")
-		(at 79.93 147.33)
+		(at 63 89.34)
 		(descr "5.0mm x 5.0mm Addressable RGB LED NeoPixel, https://cdn-shop.adafruit.com/datasheets/WS2812B.pdf")
 		(tags "LED RGB NeoPixel PLCC-4 5050")
@@
 	(footprint "LED_SMD:LED_WS2812B_PLCC4_5.0x5.0mm_P3.2mm"
 		(layer "F.Cu")
-		(at 79.93 107.61)
+		(at 63 49.62)
 		(descr "5.0mm x 5.0mm Addressable RGB LED NeoPixel, https://cdn-shop.adafruit.com/datasheets/WS2812B.pdf")
 		(tags "LED RGB NeoPixel PLCC-4 5050")
@@
 	(footprint "LED_SMD:LED_WS2812B_PLCC4_5.0x5.0mm_P3.2mm"
 		(layer "F.Cu")
-		(at 79.93 127.47)
+		(at 63 69.48)
 		(descr "5.0mm x 5.0mm Addressable RGB LED NeoPixel, https://cdn-shop.adafruit.com/datasheets/WS2812B.pdf")
 		(tags "LED RGB NeoPixel PLCC-4 5050")

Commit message: designing
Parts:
- removed D1, D10, D100, D101, D102, D103, D104, D105, D106, D107, D108, D109, D11, D110, D111, D112, D113, D114, D115, D116, D117, D118, D119, D12, D120, D121, D122, D123, D124, D125, D126, D127, D128, D129, D13, D130, D131, D132, D133, D134, D135, D136, D137, D138, D139, D14, D140, D141, D142, D143, D144, D145, D146, D147, D148, D149, D15, D150, D151, D152, D153, D154, D155, D156, D157, D158, D159, D16, D160, D161, D162, D163, D164, D165, D166, D167, D168, D169, D17, D170, D171, D172, D173, D174, D175, D176, D177, D178, D179, D18, D180, D181, D182, D183, D184, D185, D186, D187, D188, D189, D19, D190, D191, D192, D193, D194, D195, D196, D197, D198, D199, D2, D20, D200, D201, D202, D203, D204, D205, D206, D207, D208, D209, D21, D210, D211, D212, D213, D214, D215, D216, D217, D218, D219, D22, D220, D221, D222, D223, D224, D225, D226, D227, D228, D229, D23, D230, D231, D232, D233, D234, D235, D236, D237, D238, D239, D24, D240, D241, D242, D243, D244, D245, D246, D247, D248, D249, D25, D250, D251, D252, D253, D254, D255, D256, D26, D27, D28, D29, D3, D30, D31, D32, D33, D34, D35, D36, D37, D38, D39, D4, D40, D41, D42, D43, D44, D45, D46, D47, D48, D49, D5, D50, D51, D52, D53, D54, D55, D56, D57, D58, D59, D6, D60, D61, D62, D63, D64, D65, D66, D67, D68, D69, D7, D70, D71, D72, D73, D74, D75, D76, D77, D78, D79, D8, D80, D81, D82, D83, D84, D85, D86, D87, D88, D89, D9, D90, D91, D92, D93, D94, D95, D96, D97, D98, D99: WS2812B, LED_SMD:LED_WS2812B_PLCC4_5.0x5.0mm_P3.2mm
- removed TP1, TP2, TP3, TP4, TP5, TP6: TestPoint, Pegoku:TestPoint
